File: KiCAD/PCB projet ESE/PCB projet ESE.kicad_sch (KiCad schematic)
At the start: 18 parts, among them U1 STM32WB55CEUx, U2 ADXL343, U3 ZXBM5210-SP, Y1 32M

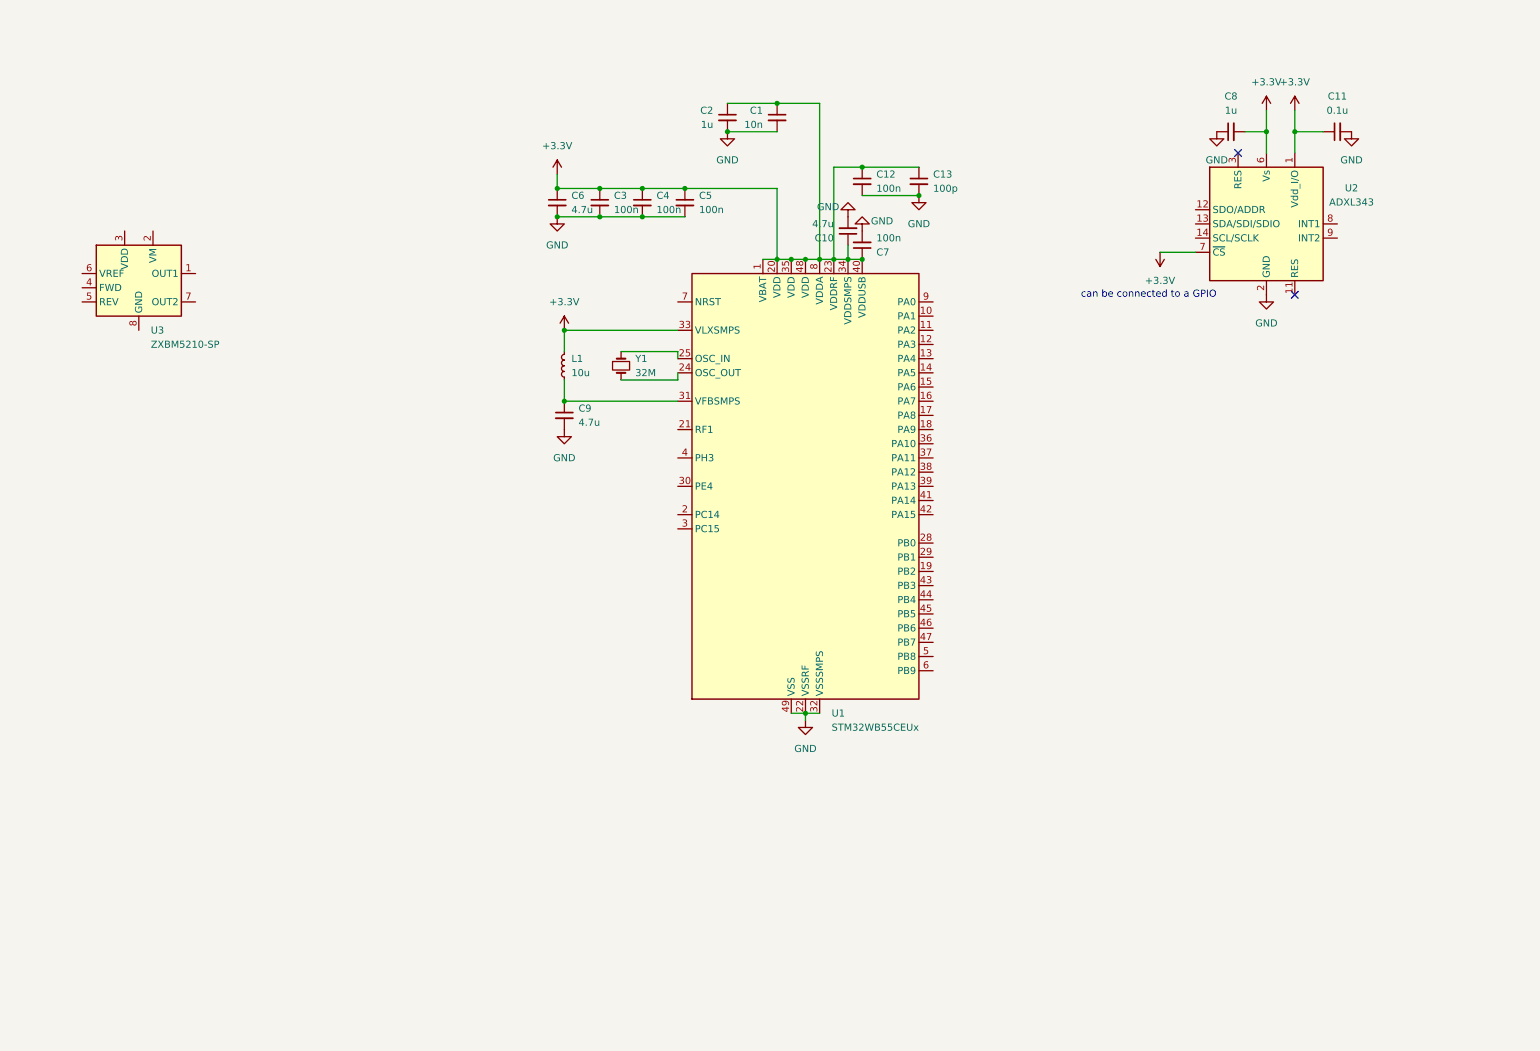
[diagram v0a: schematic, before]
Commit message: maj schematic
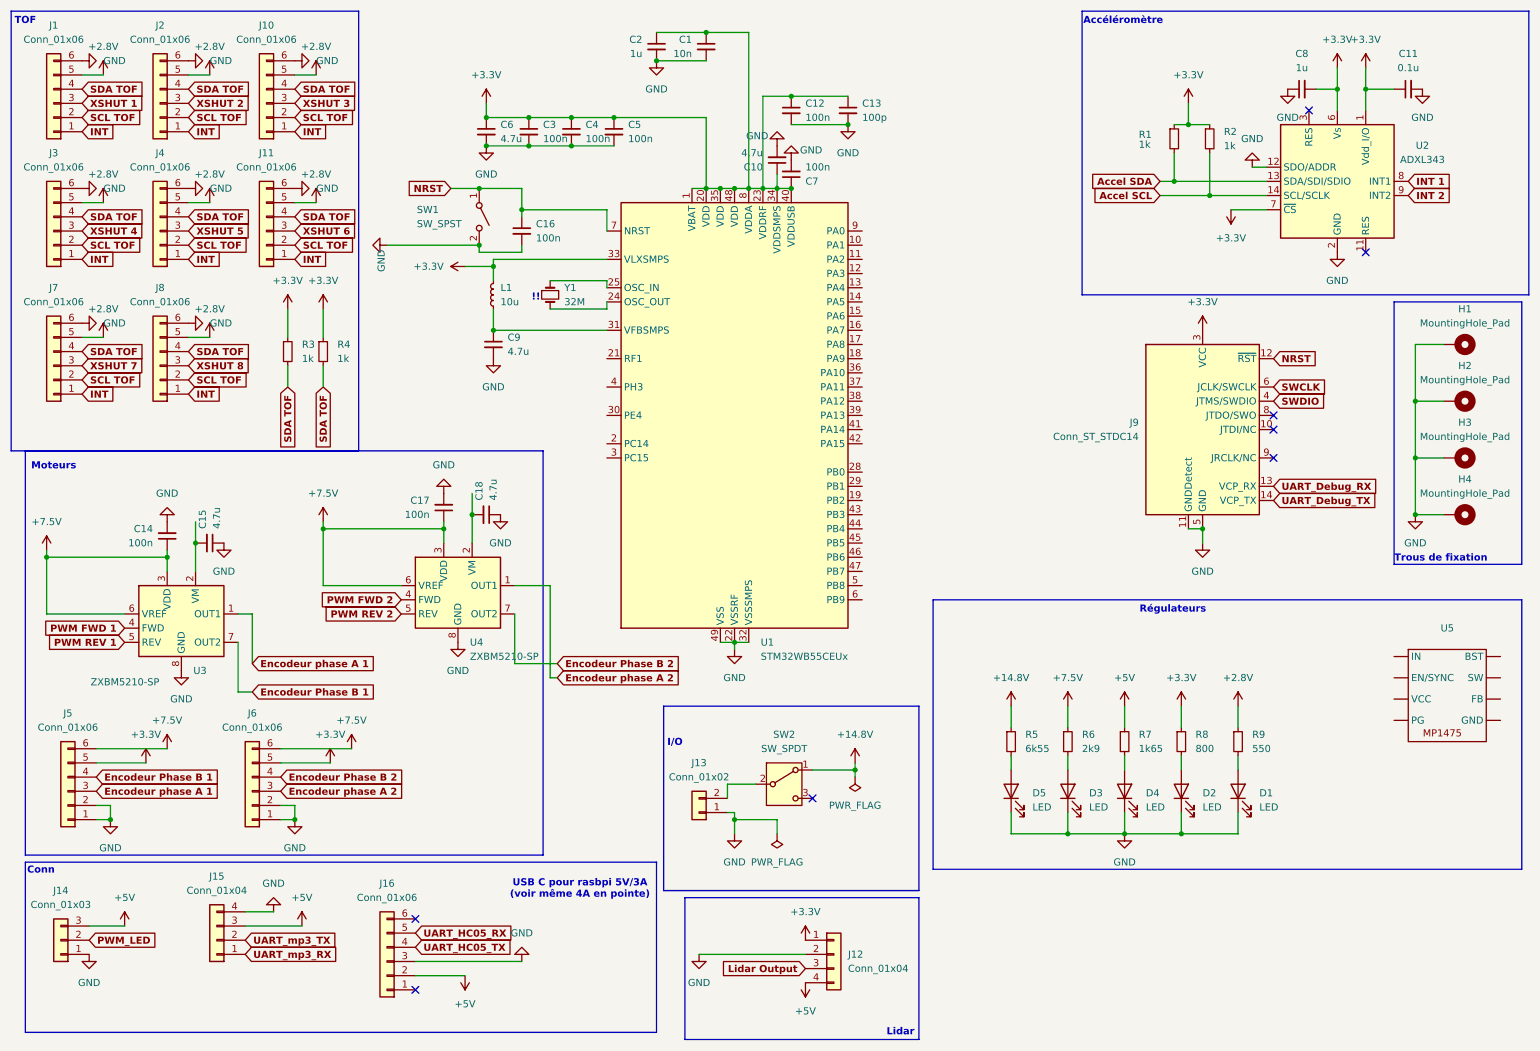
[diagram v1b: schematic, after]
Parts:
- added C14, C16, C17: 100n, symbol Device:C_Small
- added C15, C18: 4.7u, symbol Device:C_Small
- added D1, D2, D3, D4, D5: LED, symbol Device:LED
- added H1, H2, H3, H4: MountingHole_Pad, symbol Mechanical:MountingHole_Pad
- added J1, J10, J11, J16, J2, J3, J4, J5, J6, J7, J8: Conn_01x06, symbol Connector_Generic:Conn_01x06
- added J12, J15: Conn_01x04, symbol Connector_Generic:Conn_01x04
- added J13: Conn_01x02, symbol Connector_Generic:Conn_01x02
- added J14: Conn_01x03, symbol Connector_Generic:Conn_01x03
- added J9: Conn_ST_STDC14, symbol Connector:Conn_ST_STDC14
- added R1, R2, R3, R4: 1k, symbol Device:R_Small
- added R5: 6k55, symbol Device:R_Small
- added R6: 2k9, symbol Device:R_Small
- added R7: 1k65, symbol Device:R_Small
- added R8: 800, symbol Device:R_Small
- added R9: 550, symbol Device:R_Small
- added SW1: SW_SPST, symbol Switch:SW_SPST
- added SW2: SW_SPDT, symbol Switch:SW_SPDT
- added U4: ZXBM5210-SP, Package_SO:Diodes_SO-8EP, symbol Driver_Motor:ZXBM5210-SP
- added U5: ~, symbol ESE:MP1475
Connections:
- net +3.3V: now also J12.1 (Pin_1), J5.5 (Pin_5), J6.5 (Pin_5), J9.3 (VCC), R1.1, R2.1, R3.1, R4.1, R8.1
- net GND: now also U2.12 (SDO/ADDR), U3.8 (GND), U3.9 (GND), C14.2, C15.1, C16.2, C17.2, C18.1, D1.1 (K), D2.1 (K), D3.1 (K), D4.1 (K), D5.1 (K), H1.1, H2.1, H3.1, H4.1, J1.6 (Pin_6), J10.6 (Pin_6), J11.6 (Pin_6), J12.2 (Pin_2), J13.1 (Pin_1), J14.1 (Pin_1), J15.4 (Pin_4), J16.3 (Pin_3), J2.6 (Pin_6), J3.6 (Pin_6), J4.6 (Pin_6), J5.1 (Pin_1), J5.2 (Pin_2), J6.1 (Pin_1), J6.2 (Pin_2), J7.6 (Pin_6), J8.6 (Pin_6), J9.11 (GNDDetect), J9.5 (GND), J9.7 (GND), SW1.2 (B), U4.8 (GND), U4.9 (GND)
- net NRST: now reaches U1.7 (NRST)
- net NRST: now also C16.1, J9.12 (~{RST}), SW1.1 (A)
- net Encodeur phase A 1: now reaches U3.1 (OUT1)
- net Encodeur phase A 1: now also J5.3 (Pin_3)
- net at U3.2 (VM): now also C15.2
- net +7.5V: now reaches U3.3 (VDD)
- net +7.5V: now also U3.6 (VREF), C14.1, C17.1, J5.6 (Pin_6), J6.6 (Pin_6), R6.1, U4.3 (VDD), U4.6 (VREF)
- net PWM FWD 1: now reaches U3.4 (FWD)
- net PWM REV 1: now reaches U3.5 (REV)
- net Encodeur Phase B 1: now reaches U3.7 (OUT2)
- net Encodeur Phase B 1: now also J5.4 (Pin_4)
- net Accel SDA: now reaches U2.13 (SDA/SDI/SDIO)
- net Accel SDA: now also R1.2
- net Accel SCL: now reaches U2.14 (SCL/SCLK)
- net Accel SCL: now also R2.2
- net INT 1: now reaches U2.8 (INT1)
- net INT 2: now reaches U2.9 (INT2)
- new net: C18.2, U4.2 (VM)
- new net: D1.2 (A), R9.2
- new net: D4.2 (A), R7.2
- new net: D5.2 (A), R5.2
- new net: J13.2 (Pin_2), SW2.2 (B)
- new net: D2.2 (A), R8.2
- new net: D3.2 (A), R6.2
- new net +14.8V: R5.1, SW2.1 (A)
- new net +2.8V: J1.5 (Pin_5), J10.5 (Pin_5), J11.5 (Pin_5), J2.5 (Pin_5), J3.5 (Pin_5), J4.5 (Pin_5), J7.5 (Pin_5), J8.5 (Pin_5), R9.1
- new net +5V: J12.4 (Pin_4), J14.3 (Pin_3), J15.3 (Pin_3), J16.2 (Pin_2), R7.1
- new net Encodeur Phase B 2: J6.4 (Pin_4), U4.7 (OUT2)
- new net Encodeur phase A 2: J6.3 (Pin_3), U4.1 (OUT1)
- new net INT: J1.1 (Pin_1), J10.1 (Pin_1), J11.1 (Pin_1), J2.1 (Pin_1), J3.1 (Pin_1), J4.1 (Pin_1), J7.1 (Pin_1), J8.1 (Pin_1)
- new net Lidar Output : J12.3 (Pin_3)
- new net PWM FWD 2: U4.4 (FWD)
- new net PWM REV 2: U4.5 (REV)
- new net PWM_LED: J14.2 (Pin_2)
- new net SCL TOF: J1.2 (Pin_2), J10.2 (Pin_2), J11.2 (Pin_2), J2.2 (Pin_2), J3.2 (Pin_2), J4.2 (Pin_2), J7.2 (Pin_2), J8.2 (Pin_2)
- new net SDA TOF: J1.4 (Pin_4), J10.4 (Pin_4), J11.4 (Pin_4), J2.4 (Pin_4), J3.4 (Pin_4), J4.4 (Pin_4), J7.4 (Pin_4), J8.4 (Pin_4), R3.2, R4.2
- new net SWCLK: J9.6 (JCLK/SWCLK)
- new net SWDIO: J9.4 (JTMS/SWDIO)
- new net UART_Debug_RX: J9.13 (VCP_RX)
- new net UART_Debug_TX: J9.14 (VCP_TX)
- new net UART_HC05_RX: J16.5 (Pin_5)
- new net UART_HC05_TX: J16.4 (Pin_4)
- new net UART_mp3_RX: J15.1 (Pin_1)
- new net UART_mp3_TX: J15.2 (Pin_2)
- new net XSHUT 1: J1.3 (Pin_3)
- new net XSHUT 2: J2.3 (Pin_3)
- new net XSHUT 3: J10.3 (Pin_3)
- new net XSHUT 4: J3.3 (Pin_3)
- new net XSHUT 5: J4.3 (Pin_3)
- new net XSHUT 6: J11.3 (Pin_3)
- new net XSHUT 7: J7.3 (Pin_3)
- new net XSHUT 8: J8.3 (Pin_3)
- no-connect marks 2 -> 8
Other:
- note added: "!!"
- note added: "Accéléromètre"
- note added: "Conn"
- note added: "I/O"
- note added: "Lidar"
- note added: "Moteurs"
- note added: "Régulateurs"
- note added: "TOF"
- note added: "Trous de fixation"
- note added: "USB C pour rasbpi 5V/3A (voir même 4A en pointe)"
- note removed: "can be connected to a GPIO"
- moved on the sheet: C1, C10, C11, C12, C13, C2, C3, C4, C5, C6, C7, C8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
